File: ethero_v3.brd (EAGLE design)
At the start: 26 parts, among them IC1 ENC28J60SP, IC3 LP2950Z, X2 JP011821U

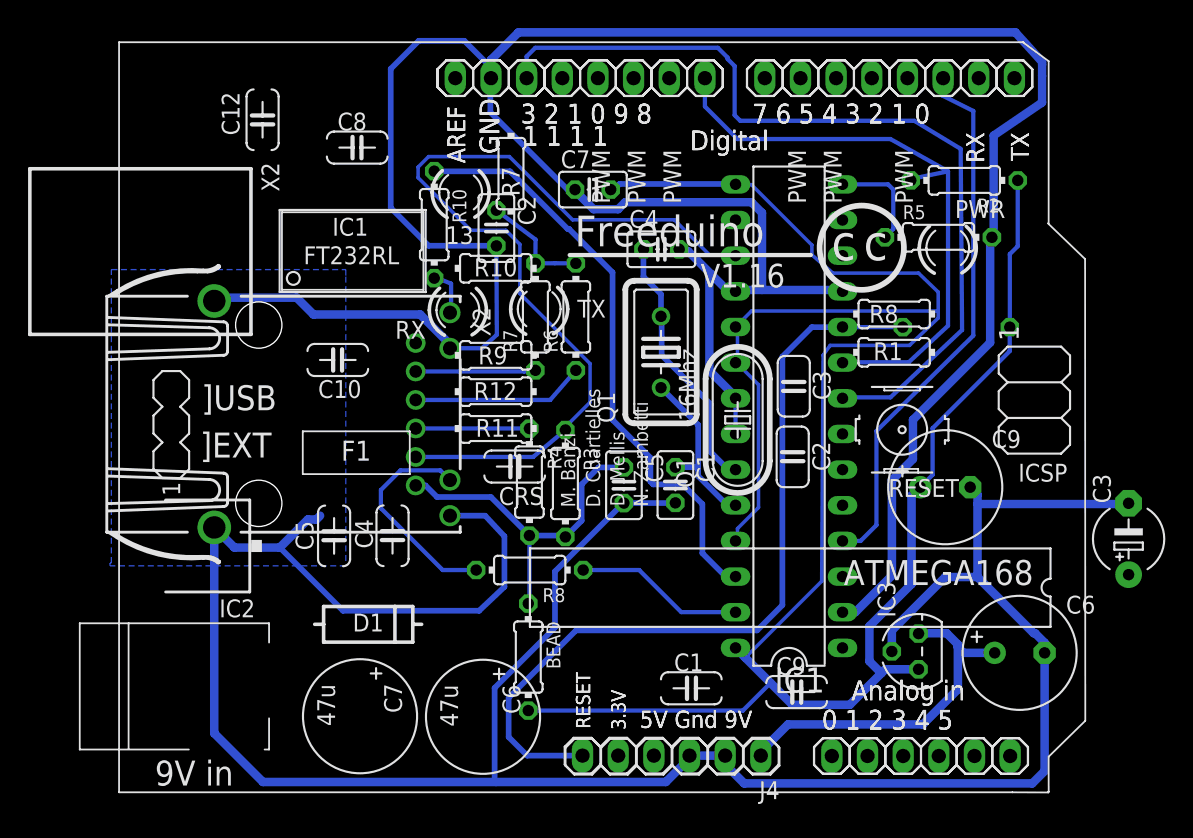
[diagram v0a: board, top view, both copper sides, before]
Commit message: version 3 ready for testing
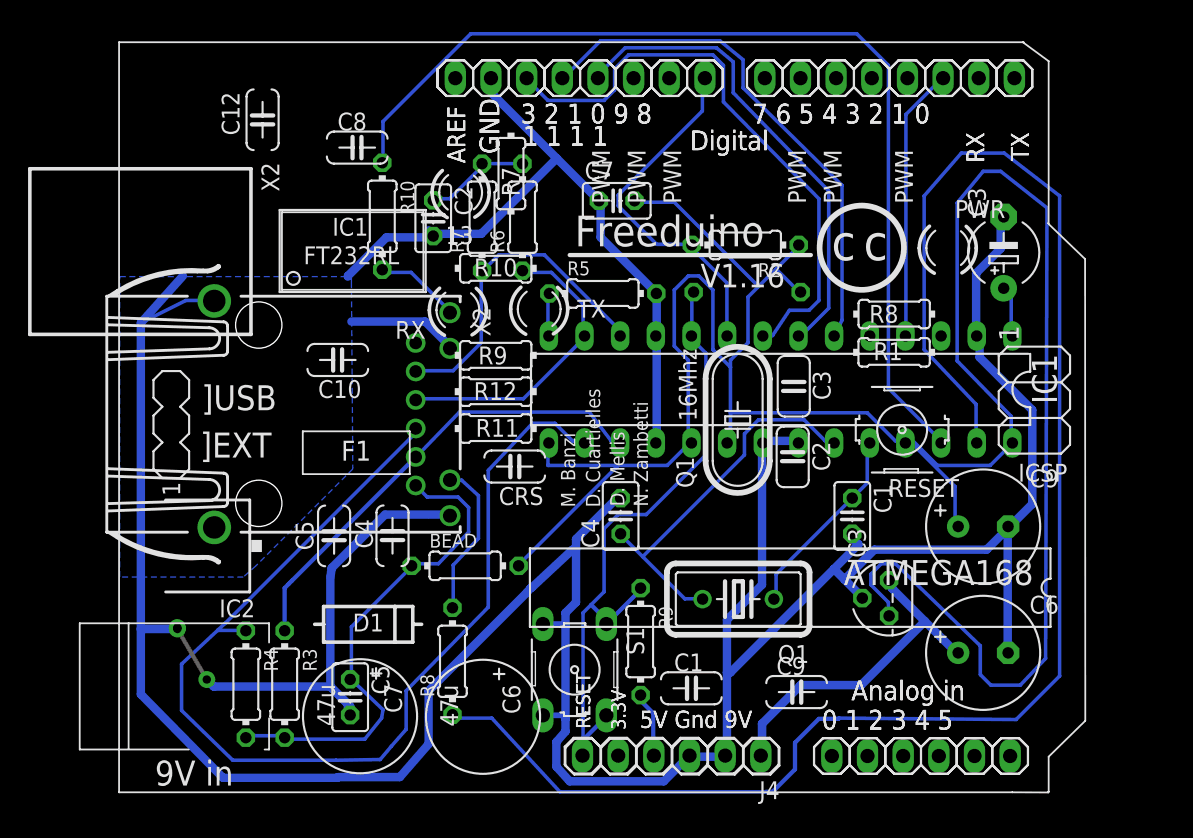
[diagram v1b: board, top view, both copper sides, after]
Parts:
- added R9: 10k, resistor:0204/7
- added S1: (no value), switch-omron:B3F-10XX
- moved R4 24.8 mm to (8.98, 7.67)
- moved C5 24.7 mm to (16.4, 6.74)
- moved R3 24.6 mm to (11.7, 7.67)
- moved R5 24.2 mm to (34.4, 35.5)
- moved C3 22.3 mm to (63.0, 38.4)
- moved C4 19.2 mm to (35.7, 19.6), turned to 90 degrees
- moved Q1 18.4 mm to (44.1, 13.7), turned to 180 degrees
- moved R2 16.3 mm to (44.6, 39.0)
- moved R1 15.1 mm to (44.7, 35.6)
- moved C1 12.8 mm to (52.2, 19.7)
- moved R8 8.51 mm to (23.7, 9.30), turned to 90 degrees
- moved R6 8.05 mm to (28.7, 40.9)
- moved R7 8.05 mm to (25.8, 40.9)
- moved BEAD 7.91 mm to (24.6, 16.1), turned to 0 degrees
- moved C2 4.55 mm to (22.3, 40.9)
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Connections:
- net DCV: now also R9.2
- net GND: now also S1.3, S1.4
- net RESET: now also R9.1, S1.1, S1.2
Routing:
- net LEDA: track 12.1 -> 115.7 mm
- net GND: track 383.9 -> 306.9 mm, vias 0 -> 2
- net TPOUTM: track 8.10 -> 77.4 mm
- net MISO: track 0.00 -> 37.2 mm
- net MOSI/OC2: track 0.00 -> 34.3 mm
- net TPOUTP: track 63.2 -> 33.2 mm
- net LEDB: track 42.6 -> 70.9 mm
- net INT0: track 39.1 -> 19.5 mm
- net SCK: track 60.9 -> 42.0 mm
- net V3.3: track 167.6 -> 185.7 mm
- net SS/OC1B: track 43.3 -> 25.6 mm
- net TPINM: track 8.53 -> 23.6 mm
- net RESET: track 58.0 -> 46.1 mm
- net CT: track 24.8 -> 35.8 mm
- net TPINP: track 12.4 -> 21.6 mm
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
